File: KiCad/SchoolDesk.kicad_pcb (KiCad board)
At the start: 2 copper layers, 99.7 x 35.6 mm, 16 parts, among them J1 Conn_1x5, J2 DIN-5_180degree, J3 Conn_1x1, J4 Conn_01x14_Female, J5 Conn_01x14_Female, J6 Conn_1x5

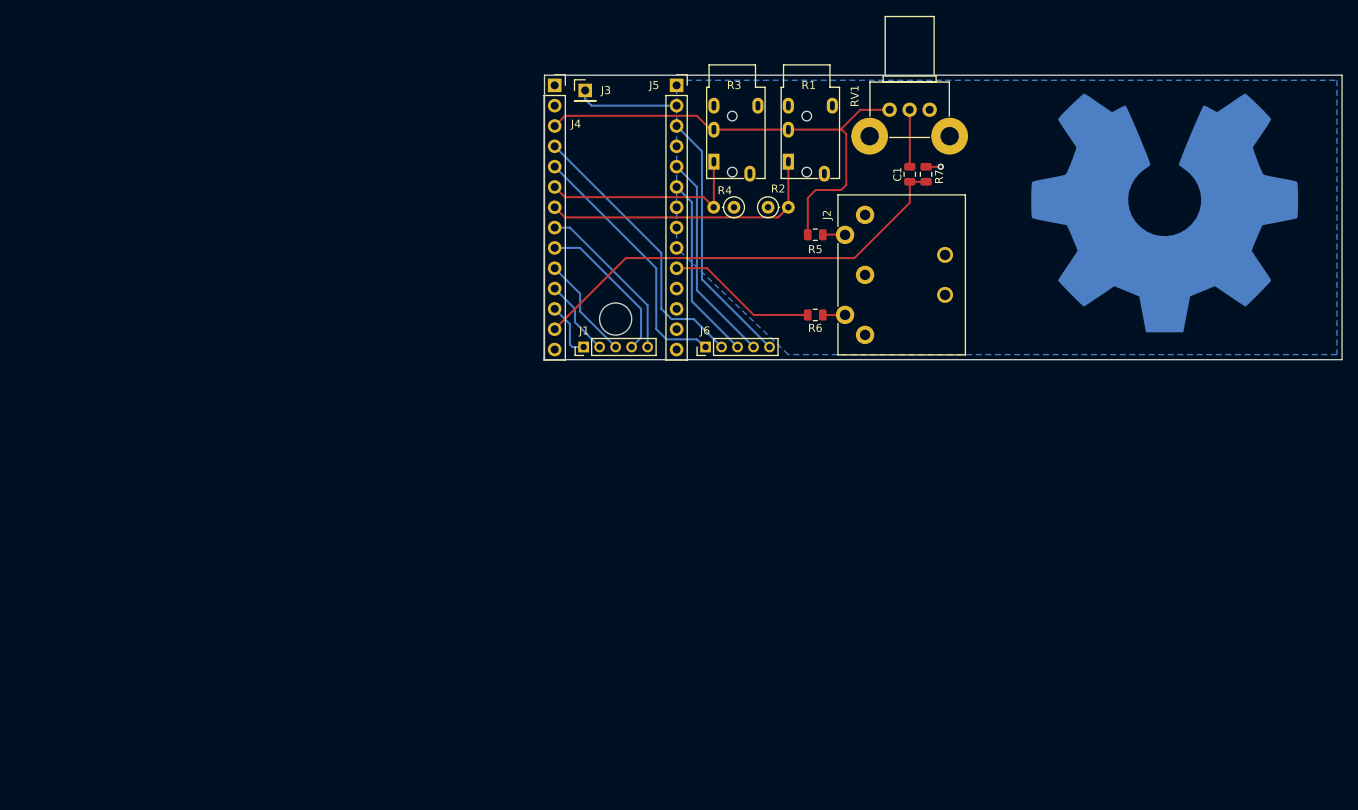
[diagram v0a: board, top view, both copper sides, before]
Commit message: First (untested) commit including PCB files.
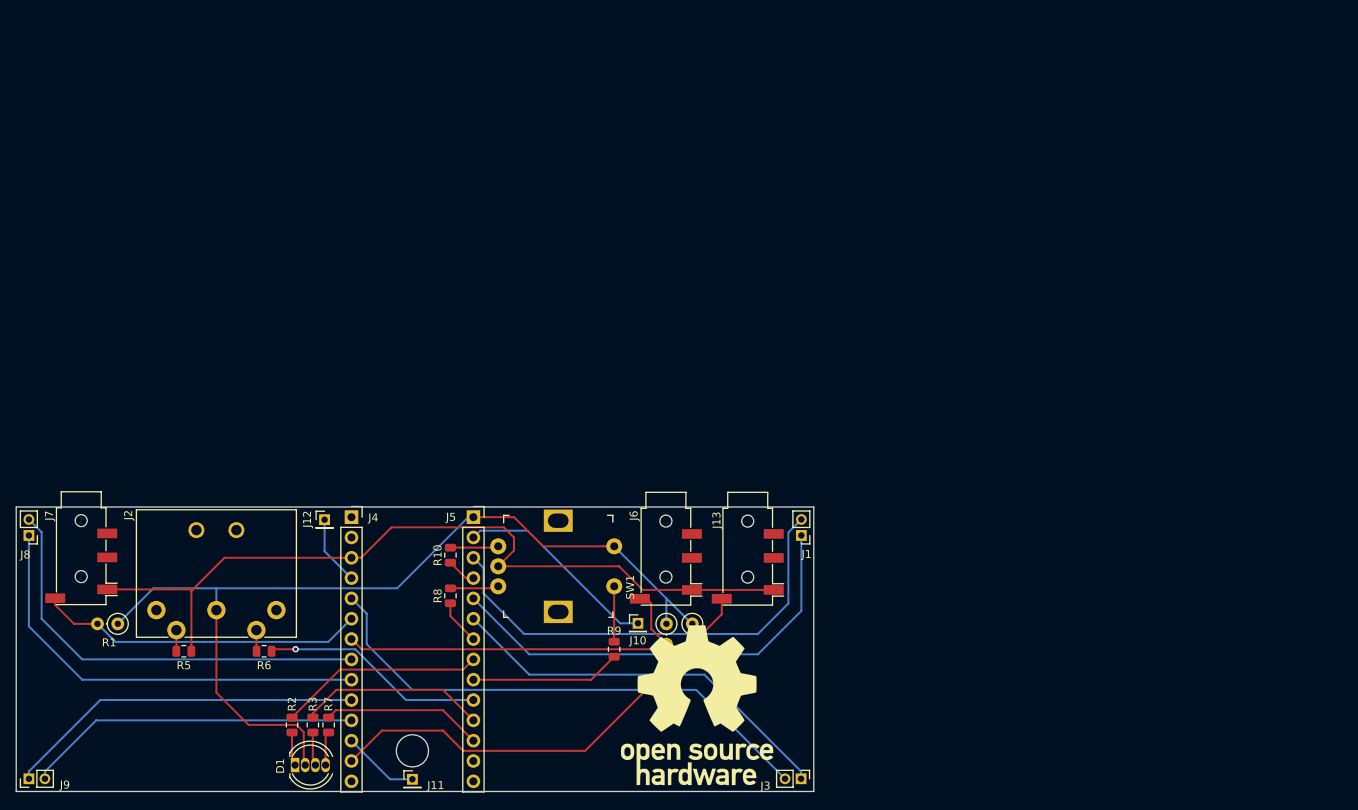
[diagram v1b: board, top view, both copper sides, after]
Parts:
- removed C1: 10uF, C_SMD_3D:C_0805_2012Metric
- removed the REF*** at (168.9, 114.3)
- removed RV1: 10k, Potentiometers:Potentiometer_Alps_RK09K_Vertical
- added D1: LED_RCBG, LED_THT_3D:LED_D5.0mm-4_RGB, F.Cu at (60.3, 183.4)
- added J10: 1x1, Pin_Headers:Pin_Header_Straight_1x01_Pitch2.00mm, F.Cu at (103.1, 165.7)
- added J11: 1x1, Pin_Headers:Pin_Header_Straight_1x01_Pitch2.00mm, F.Cu at (74.9, 185.2)
- added J12: 1x1, Pin_Headers:Pin_Header_Straight_1x01_Pitch2.00mm, F.Cu at (63.9, 152.7)
- added J13: AudioJack4, Conn_Aud_3D:Jack_3.5mm_PJ320D_Horizontal, F.Cu at (116.8, 157.7)
- added J7: AudioJack4, Conn_Aud_3D:Jack_3.5mm_PJ320D_Horizontal, F.Cu at (33.5, 157.6)
- added J8: 1x02, Pin_Headers:Pin_Header_Straight_1x02_Pitch2.00mm, F.Cu at (27.0, 154.7)
- added J9: 1x2, Pin_Headers:Pin_Header_Straight_1x02_Pitch2.00mm, F.Cu at (27.0, 185.1)
- added R10: 10k, R_SMD_3D:R_0805_2012Metric, F.Cu at (79.7, 157.1)
- added R11: 10k, Resistors_ThroughHole:R_Axial_DIN0207_L6.3mm_D2.5mm_P2.54mm_Vertical, F.Cu at (109.9, 165.7)
- added R8: 10k, R_SMD_3D:R_0805_2012Metric, F.Cu at (79.7, 162.2)
- added R9: 10k, R_SMD_3D:R_0805_2012Metric, F.Cu at (100.1, 168.9)
- added REF***: OSHW-Logo_19x20mm_SilkScreen, Symbols:OSHW-Logo_19x20mm_SilkScreen, F.Cu at (110.5, 175.9)
- added REF***: OSHW-Logo_19x20mm_SilkScreen, Symbols:OSHW-Logo_19x20mm_SilkScreen, B.Cu at (110.5, 175.9)
- added SW1: Rotary_Encoder_Switch, digikey-footprints:Rotary_Encoder_Switched_PEC11R, F.Cu at (93.2, 152.8)
- J1: value Conn_1x5 -> 1x2; footprint Pin_Headers:Pin_Header_Straight_1x05_Pitch2.00mm -> Pin_Headers:Pin_Header_Straight_1x02_Pitch2.00mm
- J3: value Conn_1x1 -> 1x2; footprint P_2.54_3D:PinHeader_1x01_P2.54mm_Vertical -> Pin_Headers:Pin_Header_Straight_1x02_Pitch2.00mm
- J6: value Conn_1x5 -> AudioJack4; footprint Pin_Headers:Pin_Header_Straight_1x05_Pitch2.00mm -> Conn_Aud_3D:Jack_3.5mm_PJ320D_Horizontal
- R1: value R_FSR -> 10k; footprint Connectors:PJ320E_3.5mm_Jack -> Resistors_ThroughHole:R_Axial_DIN0207_L6.3mm_D2.5mm_P2.54mm_Vertical
- R2: value 10k -> 330; footprint Resistors_ThroughHole:R_Axial_DIN0207_L6.3mm_D2.5mm_P2.54mm_Vertical -> R_SMD_3D:R_0805_2012Metric
- R3: value R_FSR -> 330; footprint Connectors:PJ320E_3.5mm_Jack -> R_SMD_3D:R_0805_2012Metric
- R7: value 47k -> 330
- moved R1 101.8 mm to (38.1, 165.7), turned to 180 degrees
- moved J2 101.4 mm to (42.9, 164.0), turned to 0 degrees
- moved R7 100.1 mm to (64.5, 178.4), turned to 90 degrees
- moved R5 94.6 mm to (46.4, 169.2), turned to 180 degrees
- moved J3 90.2 mm to (123.5, 185.1), turned to 270 degrees
- moved R2 87.9 mm to (59.9, 178.4), turned to 90 degrees
- moved R3 86.4 mm to (62.5, 178.4), turned to 90 degrees
- moved R6 80.7 mm to (56.4, 169.2)
- moved J4 59.7 mm to (67.3, 152.4)
- moved J5 59.7 mm to (82.5, 152.4)
- moved R4 52.8 mm to (106.7, 165.7), turned to 270 degrees
- moved J1 36.0 mm to (123.5, 154.7), turned to 180 degrees
- moved J6 27.0 mm to (106.6, 157.7), turned to 270 degrees
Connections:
- J2 pad 2: (no net) -> GND
- J4 pad 10: Net-(J1-Pad3) -> Net-(J4-Pad10)
- J4 pad 11: Net-(J1-Pad2) -> Net-(J4-Pad11)
- J4 pad 12: Net-(J1-Pad1) -> Net-(J11-Pad1)
- J4 pad 13: Net-(C1-Pad1) -> Net-(J13-PadS)
- J4 pad 3: Net-(J4-Pad3) -> 3.3v
- J4 pad 4: Net-(J4-Pad4) -> Net-(J12-Pad1)
- J4 pad 5: Net-(J4-Pad5) -> Net-(J3-Pad2)
- J4 pad 8: Net-(J1-Pad5) -> Net-(J4-Pad8)
- J4 pad 9: Net-(J1-Pad4) -> Net-(J4-Pad9)
- J5 pad 11: (no net) -> Net-(J5-Pad11)
- J5 pad 12: (no net) -> Net-(J5-Pad12)
- J5 pad 2: Net-(J3-Pad1) -> Net-(J10-Pad1)
- J5 pad 3: Net-(J5-Pad3) -> Net-(J1-Pad2)
- J5 pad 4: (no net) -> Net-(J5-Pad4)
- J5 pad 5: Net-(J5-Pad5) -> Net-(J1-Pad1)
- J5 pad 6: Net-(J5-Pad6) -> Net-(J3-Pad1)
- J5 pad 7: (no net) -> Net-(J5-Pad7)
- J5 pad 8: (no net) -> Net-(J5-Pad8)
- J5 pad 9: (no net) -> Net-(J5-Pad9)
- R1 pad 1: Net-(J4-Pad7) -> GND
- R1 pad 2: Net-(J4-Pad3) -> Net-(J4-Pad6)
- R2 pad 1: GND -> Net-(D1-Pad1)
- R2 pad 2: Net-(J4-Pad7) -> Net-(J5-Pad8)
- R3 pad 1: Net-(J4-Pad6) -> Net-(D1-Pad3)
- R3 pad 2: Net-(J4-Pad3) -> Net-(J5-Pad11)
- R4 pad 2: Net-(J4-Pad6) -> Net-(J4-Pad7)
- R5 pad 1: Net-(J4-Pad3) -> 3.3v
- R6 pad 1: Net-(J2-Pad5) -> Net-(J5-Pad10)
- R6 pad 2: Net-(J5-Pad10) -> Net-(J2-Pad5)
- R7 pad 2: Net-(C1-Pad1) -> Net-(J5-Pad12)
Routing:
- net GND: track 1.84 -> 115.9 mm, vias 1 -> 0
- net 3.3v: track 0.00 -> 104.2 mm
- net Net-(J3-Pad2): track 0.00 -> 66.4 mm
- net Net-(J4-Pad3): track 61.4 -> 0.00 mm
- net Net-(J13-PadS): track 0.00 -> 58.0 mm
- net Net-(C1-Pad1): track 55.6 -> 0.00 mm
- net Net-(J4-Pad9): track 0.00 -> 54.5 mm
- net Net-(J4-Pad8): track 0.00 -> 53.9 mm
- net Net-(J1-Pad2): track 9.63 -> 58.9 mm
- net Net-(J1-Pad1): track 7.08 -> 55.6 mm
- net Net-(J4-Pad10): track 0.00 -> 44.9 mm
- net Net-(J4-Pad11): track 0.00 -> 41.9 mm
- net Net-(J3-Pad1): track 12.9 -> 49.8 mm
- net Net-(J4-Pad4): track 35.3 -> 0.00 mm
- net Net-(J4-Pad5): track 32.6 -> 0.00 mm
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- removed copper zone on B.Cu, net GND
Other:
- outline, holes or cut-outs redrawn
- board text added: "0 Touch"
- board text added: "Enc-A 2"
- board text added: "Enc-B 5"
- board text added: "Pedal 14"
- board text added: "Pedal 20"
- board text added: "Pedal 21"
- board text added: "Switch 7"
- board text added: "Touch 16"
- board text added: "Touch 17"
- board text added: "Touch 18"
- board text added: "Touch 19"
- board text added: "Touch 22"
- board text added: "Touch 4"
- board text removed: "16 Touch"
- board text removed: "17 Touch"
- board text removed: "18 Touch"
- board text removed: "19 Touch"
- board text removed: "22 Touch"
- board text removed: "4 Touch"
- board text removed: "POT 14"
- board text removed: "Pedal A 21"
- board text removed: "Pedal B 20"
- board text removed: "Touch 0"
